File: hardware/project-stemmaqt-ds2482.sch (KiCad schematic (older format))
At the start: 21 parts, among them J1 SM04B-SRSS-TB(LF)(SN), J2 SM04B-SRSS-TB(LF)(SN), J3 Conn_01x03_Male, J4 Conn_01x03_Male, Q1 Q_PMOS_GSD, U1 DS2482S-100+

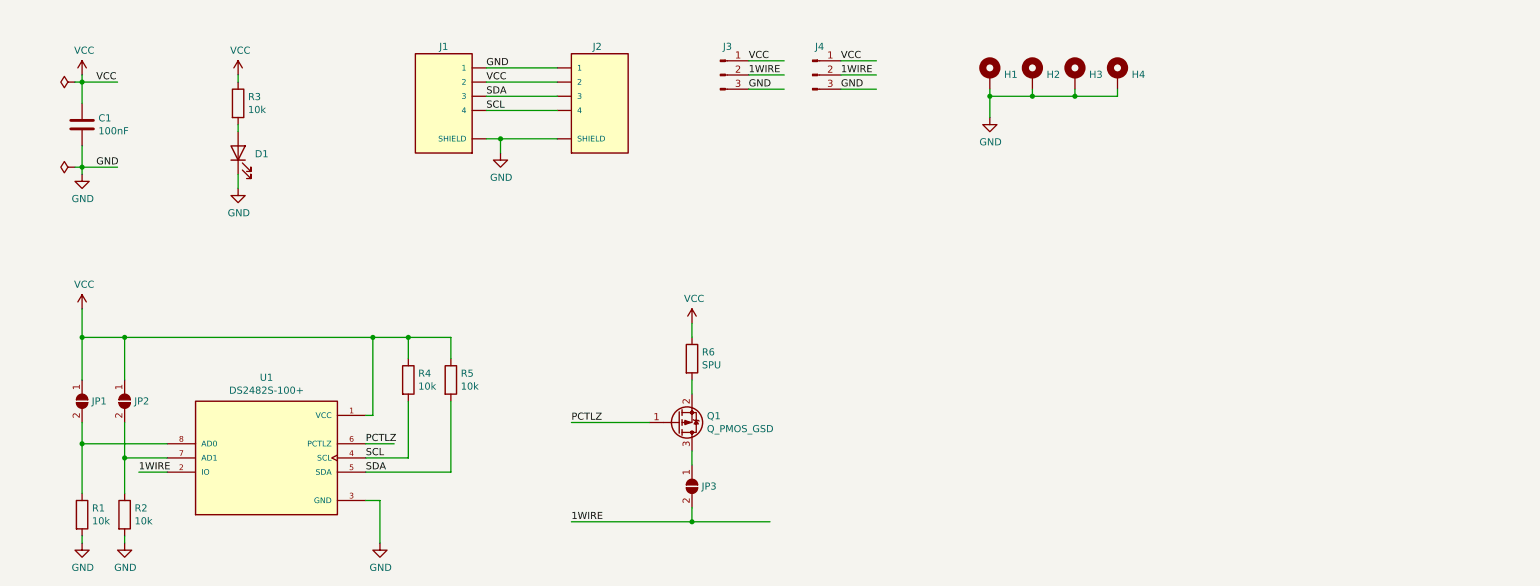
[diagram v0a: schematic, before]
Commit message: Little schematic cleanup
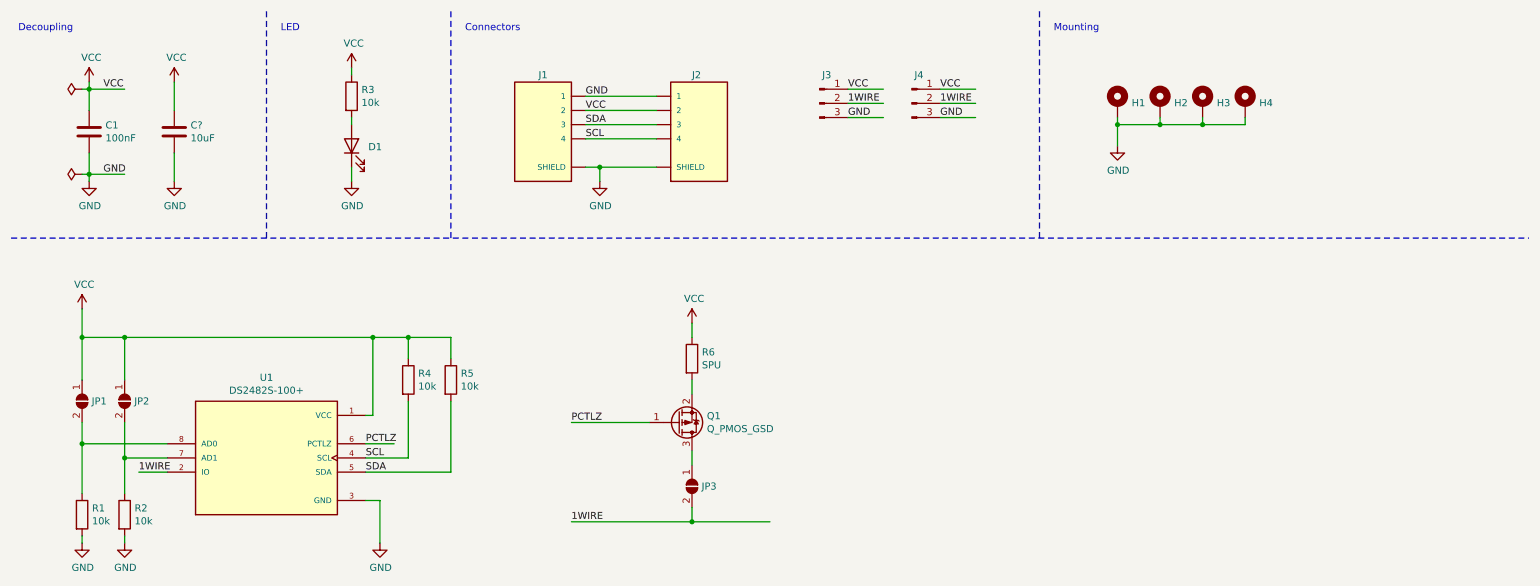
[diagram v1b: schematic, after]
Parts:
- added C?: 10uF, Capacitor_SMD:C_1210_3225Metric, symbol Device:C
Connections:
- wire segments 66 -> 68
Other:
- note added: "Connectors"
- note added: "Decoupling"
- note added: "LED"
- note added: "Mounting"
- moved on the sheet: C1, D1, H1, H2, H3, H4, J1, J2, J3, J4, R3
